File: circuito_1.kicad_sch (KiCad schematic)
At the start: 17 parts, among them J1 Conn_01x02, SW1 SW_SPDT, T1 Transformer_1P_2S, U4 LM7815_TO220, U5 LM7815_TO220

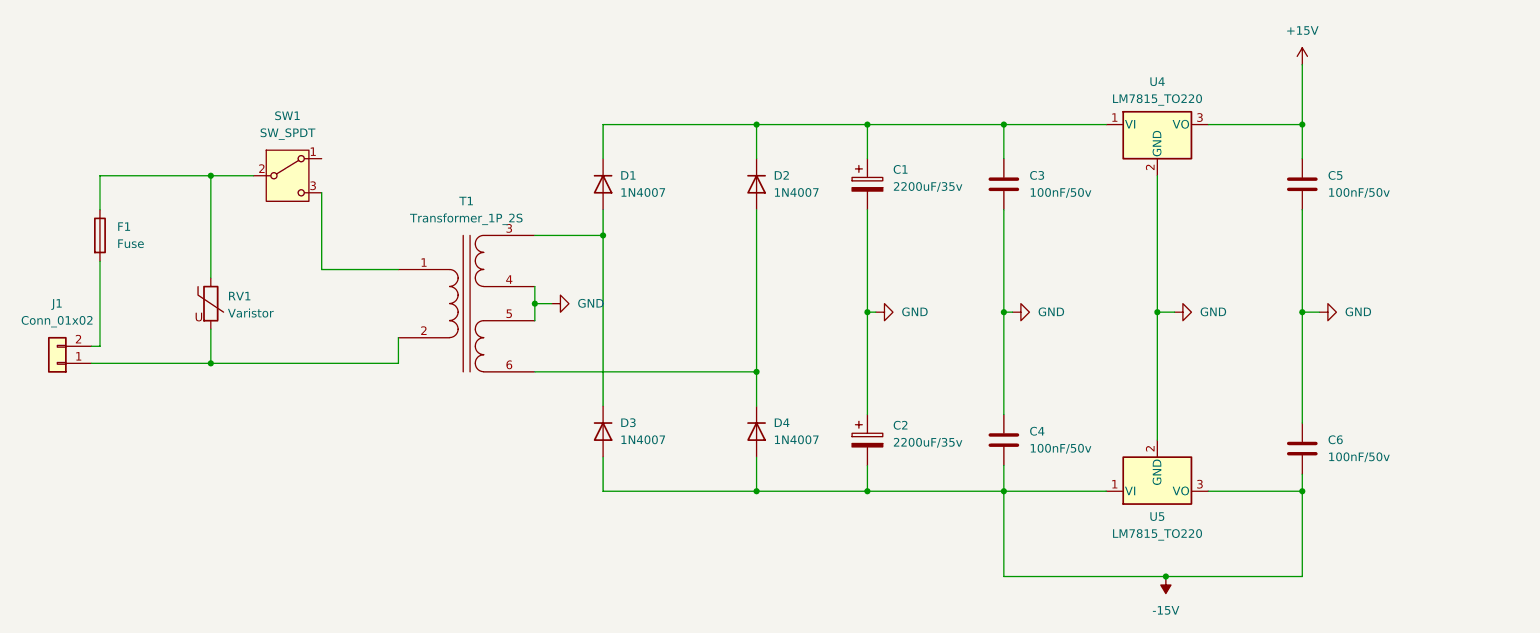
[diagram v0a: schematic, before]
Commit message: Reorganização dos esquemáticos em pages.
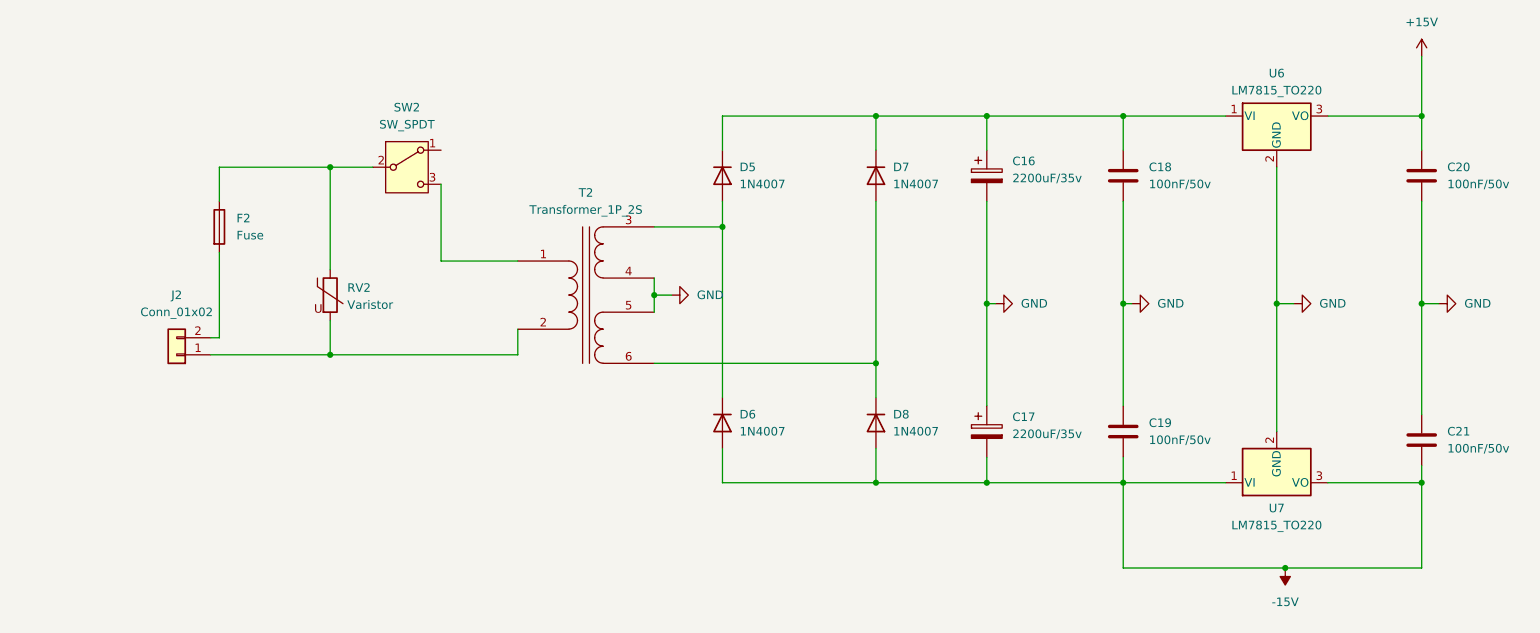
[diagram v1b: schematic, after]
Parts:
- removed C1, C2: 2200uF/35v, symbol Device:C_Polarized
- removed C3, C4, C5, C6: 100nF/50v, symbol Device:C
- removed D1, D2, D3, D4: 1N4007, Diode_THT:D_DO-41_SOD81_P10.16mm_Horizontal, symbol Diode:1N4007
- removed F1: Fuse, symbol Device:Fuse
- removed J1: Conn_01x02, symbol Connector_Generic:Conn_01x02
- removed RV1: Varistor, symbol Device:Varistor
- removed SW1: SW_SPDT, symbol Switch:SW_SPDT
- removed T1: Transformer_1P_2S, symbol Device:Transformer_1P_2S
- removed U4, U5: LM7815_TO220, Package_TO_SOT_THT:TO-220-3_Vertical, symbol Regulator_Linear:LM7815_TO220
- added C16, C17: 2200uF/35v, symbol Device:C_Polarized
- added C18, C19, C20, C21: 100nF/50v, symbol Device:C
- added D5, D6, D7, D8: 1N4007, Diode_THT:D_DO-41_SOD81_P10.16mm_Horizontal, symbol Diode:1N4007
- added F2: Fuse, symbol Device:Fuse
- added J2: Conn_01x02, symbol Connector_Generic:Conn_01x02
- added RV2: Varistor, symbol Device:Varistor
- added SW2: SW_SPDT, symbol Switch:SW_SPDT
- added T2: Transformer_1P_2S, symbol Device:Transformer_1P_2S
- added U6, U7: LM7815_TO220, Package_TO_SOT_THT:TO-220-3_Vertical, symbol Regulator_Linear:LM7815_TO220
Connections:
- net +15V: now also C20.1, U6.3 (VO)
- net -15V: now also C17.2, C19.2, C21.2, D6.2 (A), D8.2 (A), U7.1 (VI), U7.3 (VO)
- net GND: now also C16.2, C17.1, C18.2, C19.1, C20.2, C21.1, T2.4 (SB), T2.5 (SC), U6.2 (GND), U7.2 (GND)
- new net: C16.1, C18.1, D5.1 (K), D7.1 (K), U6.1 (VI)
- new net: D7.2 (A), D8.1 (K), T2.6 (SD)
- new net: J2.1 (Pin_1), RV2.2, T2.2 (AB)
- new net: F2.2, J2.2 (Pin_2)
- new net: F2.1, RV2.1, SW2.2 (B)
- new net: SW2.3 (C), T2.1 (AA)
- new net: D5.2 (A), D6.1 (K), T2.3 (SA)
